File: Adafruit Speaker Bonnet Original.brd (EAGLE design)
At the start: 65 x 30.7 mm, 31 parts, among them X1 3.5mm, X2 3.5mm, X3 4 JST-PH

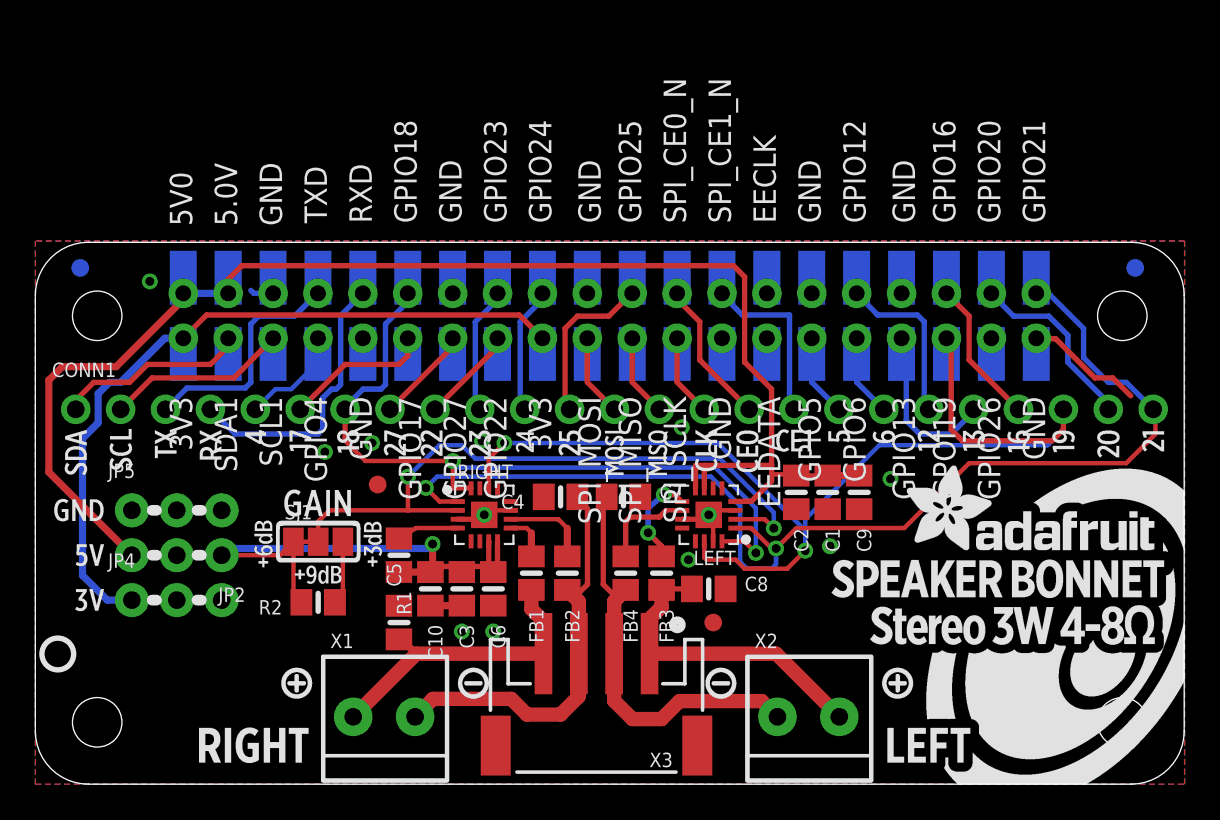
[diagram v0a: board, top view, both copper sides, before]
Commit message: Add rev C.
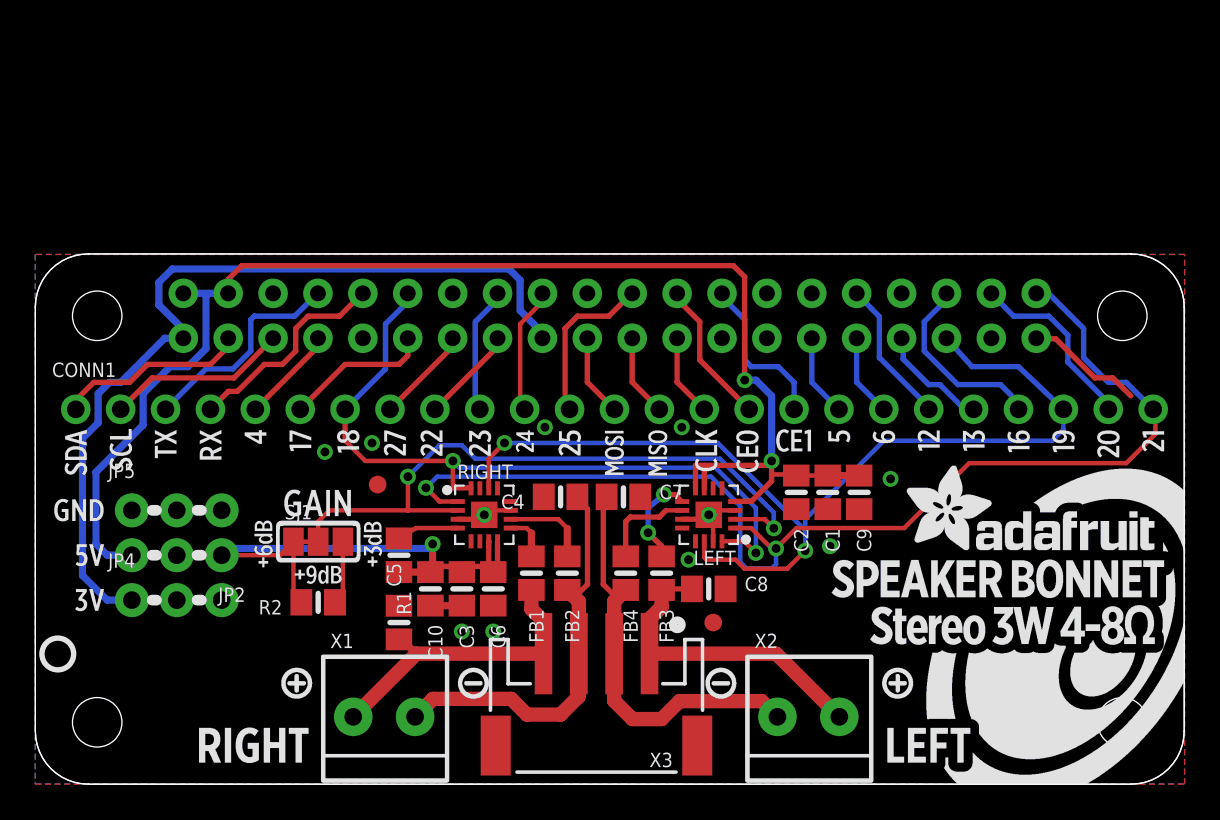
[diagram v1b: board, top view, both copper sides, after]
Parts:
- FID1, FID2: value FIDUCIAL_1MM -> FIDUCIAL""
- RPI1: value RASPBERRYPI_BPLUS_BONNET_THMSMT -> RASPBERRYPI_BPLUS_BONNETNODIM; device microbuilder:PI_BONNET_THMSMT -> microbuilder:PI_BONNET_NODIM
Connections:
- net 3.3V: no longer RPI1.S1, RPI1.S17
- net 5.0V: no longer RPI1.S2, RPI1.S4
- net BCLK: no longer RPI1.S12
- net DIN: no longer RPI1.S40
- net EECLK: no longer RPI1.S28
- net EEDATA: no longer RPI1.S27
- net GND: no longer RPI1.S14, RPI1.S20, RPI1.S25, RPI1.S30, RPI1.S34, RPI1.S39, RPI1.S6, RPI1.S9
- net GPIO12: no longer RPI1.S32
- net GPIO13: no longer RPI1.S33
- net GPIO16: no longer RPI1.S36
- net GPIO17: no longer RPI1.S11
- net GPIO20: no longer RPI1.S38
- net GPIO22: no longer RPI1.S15
- net GPIO23: no longer RPI1.S16
- net GPIO24: no longer RPI1.S18
- net GPIO25: no longer RPI1.S22
- net GPIO26: no longer RPI1.S37
- net GPIO27: no longer RPI1.S13
- net GPIO4: no longer RPI1.S7
- net GPIO5: no longer RPI1.S29
- net GPIO6: no longer RPI1.S31
- net LRCLK: no longer RPI1.S35
- net RXD: no longer RPI1.S10
- net SCL: no longer RPI1.S5
- net SDA: no longer RPI1.S3
- net SPI_CE0: no longer RPI1.S24
- net SPI_CE1: no longer RPI1.S26
- net SPI_MISO: no longer RPI1.S21
- net SPI_MOSI: no longer RPI1.S19
- net SPI_SCLK: no longer RPI1.S23
- net TXD: no longer RPI1.S8
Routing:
- net LRCLK: track 63.1 -> 57.2 mm
- net GPIO13: track 11.1 -> 6.40 mm
- net RXD: track 16.7 -> 12.1 mm
- net 3.3V: track 49.2 -> 53.8 mm
- net 5.0V: track 120.0 -> 116.9 mm, vias 1 -> 3
- net GPIO12: track 10.6 -> 8.24 mm
- net TXD: track 14.2 -> 12.4 mm
- net SPI_CE1: track 10.8 -> 9.14 mm
- net BCLK: track 43.4 -> 41.9 mm
- net GPIO4: track 6.90 -> 5.49 mm
- net GPIO16: track 9.49 -> 10.7 mm
- net SPI_MISO: track 5.55 -> 4.66 mm
- net GPIO26: track 0.89 -> 0.00 mm
- net SDA: track 11.8 -> 10.9 mm
- net SPI_SCLK: track 5.55 -> 4.66 mm
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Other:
- board size 65 x 30.7 mm -> 65 x 30 mm
